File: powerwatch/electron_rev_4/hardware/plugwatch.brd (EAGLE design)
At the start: 52.8 x 90.9 mm, 125 parts, among them J1 DM3AT-SF-PEJM5, Q1 SI223DDS, U1 BGA725L6-ALT, U10 SIP32510, U11 SN74AHC1G04DCKR, U12 SIP32510, U13 AB1815-T3, U16 MAX6746, U2 SAFFB1G56KB0F0A, U3 IRM-03-5V, U4 MAX-M8, U5 MAX9910, U6 LIS2DW12, U8 MAX9910, U9 SIP32510, X1 ABS07-32.768KHZ-7-T

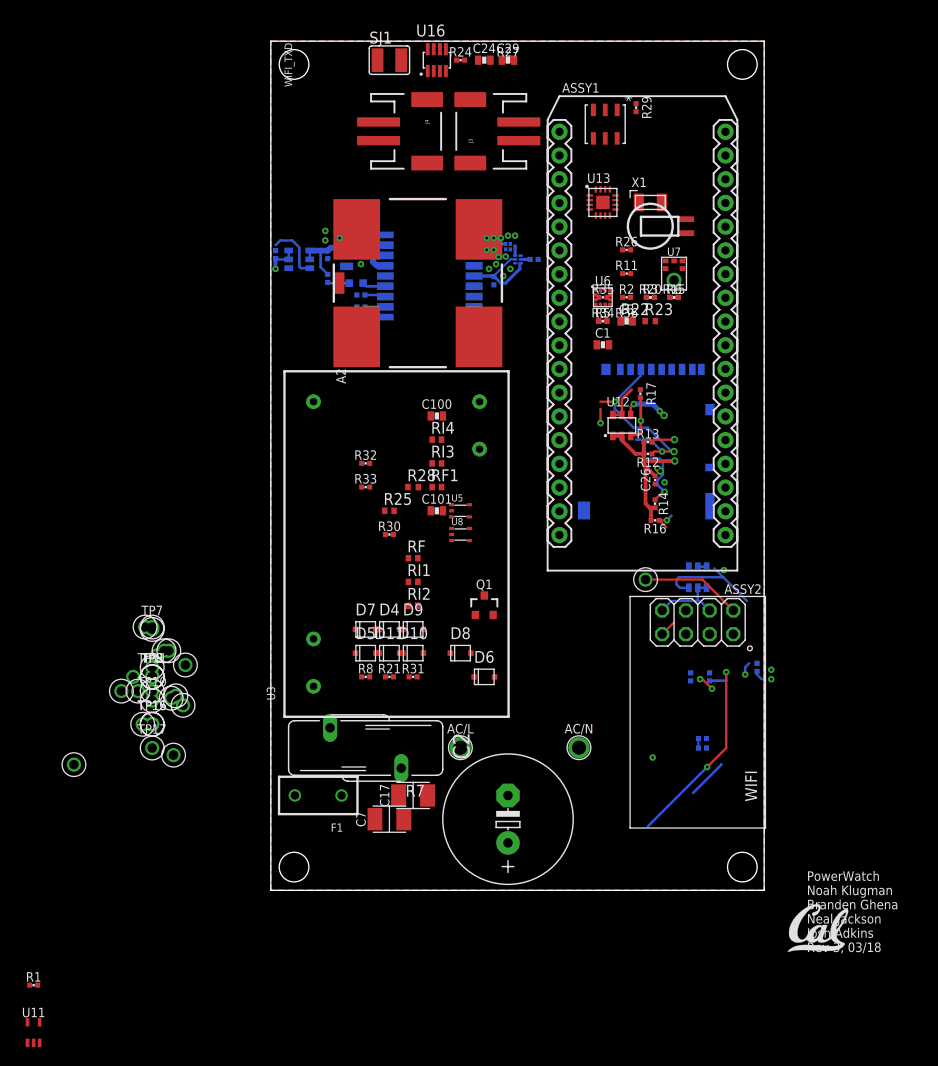
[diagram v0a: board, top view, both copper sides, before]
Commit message: doing routing
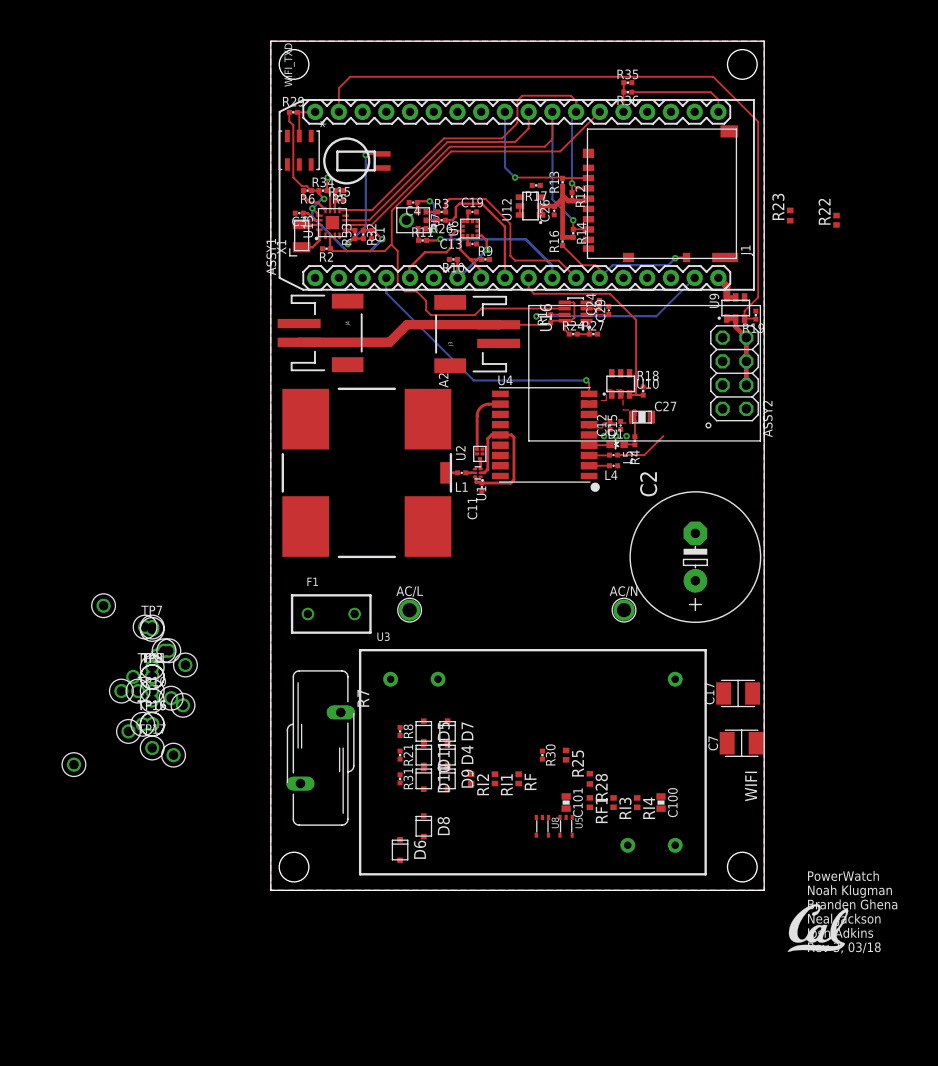
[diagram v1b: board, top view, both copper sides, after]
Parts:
- removed Q1: SI223DDS, fets:SOT23-3
- removed R20: 10k, passives:0402_RES
- removed SJ1: (no value), jumper:SJW
- removed U11: SN74AHC1G04DCKR, chips:SC70
- added C4: 1uF, passives:0402_CAP
- C1, C24, C29, C3: device passives:0603_CAP -> passives:0402_CAP
- moved R1 90.3 mm to (30.0, 61.2), turned to 90 degrees
- moved C19 62.5 mm to (21.6, 72.6), flipped to the top, turned to 0 degrees
- moved C13 58.4 mm to (21.6, 69.2), flipped to the top, turned to 0 degrees
- moved TP13 57.7 mm to (-15.2, 17.0)
- moved R10 51.4 mm to (19.6, 67.6), flipped to the top, turned to 180 degrees
- moved R9 50.7 mm to (23.0, 67.6), flipped to the top, turned to 0 degrees
- moved ASSY1 50.4 mm to (51.7, 84.6), turned to 180 degrees
- moved C100 47.9 mm to (41.8, 9.40), turned to 270 degrees
- moved RI4 44.4 mm to (39.2, 9.40), turned to 270 degrees
- moved R18 42.0 mm to (39.9, 53.5), flipped to the top
- moved RI3 41.0 mm to (36.7, 9.40), turned to 270 degrees
- moved R6 40.9 mm to (3.94, 74.9), turned to 180 degrees
- moved C7 38.6 mm to (50.4, 15.7)
- moved R19 37.7 mm to (51.9, 61.6), flipped to the top, turned to 270 degrees
- moved RF1 37.5 mm to (34.2, 9.40), turned to 270 degrees
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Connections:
- removed net !RTC_INT2: R20.2, U13.4
- removed net N$35: J4.2, Q1.3, SJ1.2
- removed net N$9: Q1.1, U11.4
- net !EXTERNAL_RST: no longer U11.2
- net GND: now also C4.2; no longer U11.3
- net N$23: now also J4.2; no longer Q1.2, SJ1.1, U11.5
- net VCC: now also C4.1; no longer R20.1
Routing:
- net WDI: track 0.00 -> 63.3 mm
- net WIFI_PWR_EN: track 12.9 -> 72.9 mm
- net WIFI_TXD: track 10.8 -> 56.0 mm
- net !RTC_INT1: track 0.00 -> 44.2 mm, vias 0 -> 1
- net WIFI_RXD: track 1.80 -> 45.2 mm
- net SD_MOSI: track 5.78 -> 44.1 mm, vias 2 -> 1
- net SD_MISO: track 6.63 -> 44.0 mm
- net N$23: track 0.00 -> 34.8 mm
- net VCC: track 10.8 -> 41.1 mm, vias 2 -> 5
- net SD_SCLK: track 0.69 -> 25.5 mm, vias 2 -> 0
- net !EXTERNAL_RST: track 0.00 -> 21.7 mm, vias 0 -> 1
- net !GPS_RESET: track 7.07 -> 28.5 mm
- net MIC_WS: track 0.00 -> 20.6 mm
- net GPS_PWR_EN: track 6.30 -> 23.6 mm
- net GPS_VCC: track 19.8 -> 3.14 mm
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- added copper zone on layer 1, net GPS_VCC
